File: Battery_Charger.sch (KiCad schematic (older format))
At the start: 48 parts, among them J8 USB_B_Micro, Q10 BC817, Q11 BC807, Q12 BSS138, Q13 BSS138, Q14 BSS138, Q9 BSS84, SW2 set_current, SW3 PWRON, U23 BQ24079RGT, U24 Holder 2x18650

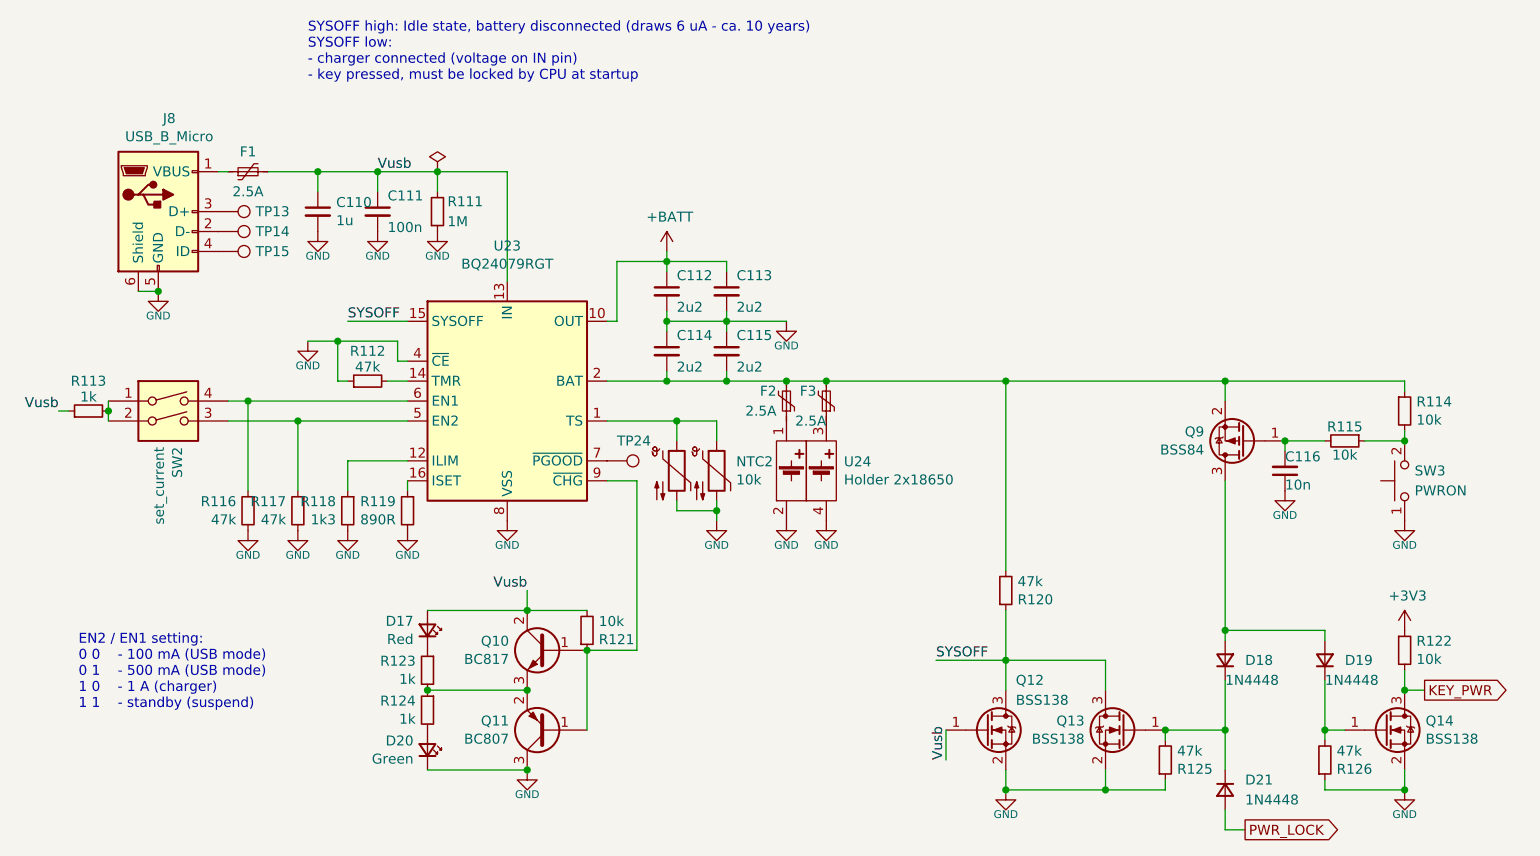
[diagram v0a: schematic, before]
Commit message: - PCB WiP
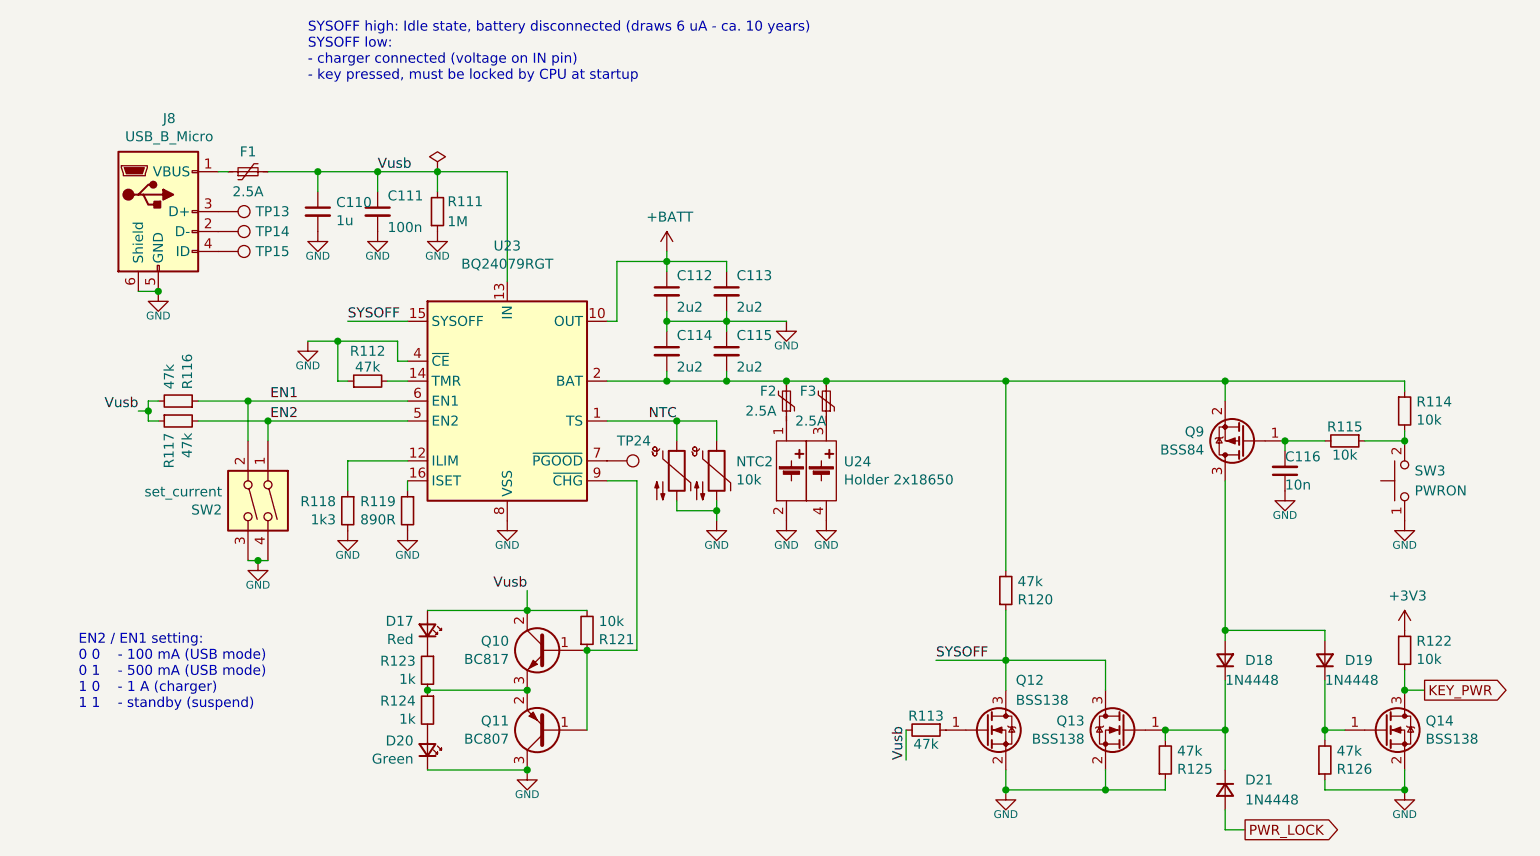
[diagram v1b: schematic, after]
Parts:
- D18, D19, D21: footprint Diode_SMD:D_SOD-323 -> miscellaneous_my:D_SOD-323-523_HandSoldering
- R113: value 1k -> 47k
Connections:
- net GND: now also SW2.3, SW2.4; no longer R116.2, R117.2
- net Vusb: now also R113.2, R116.2, R117.1; no longer Q12.1 (G), R113.1
- net NTC: now reaches NTC1.1, NTC2.1, U23.1 (TS)
- net EN1: now reaches R116.1, U23.6 (EN1)
- net EN1: now also SW2.2; no longer SW2.4
- new net: Q12.1 (G), R113.1
- new net EN2: R117.2, SW2.1, U23.5 (EN2)
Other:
- moved on the sheet: R116, R117, SW2
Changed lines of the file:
@@
 L Switch:SW_DIP_x02 SW?
 U 1 1 5F7AA902
-P 3150 3500
+P 3550 3900
 AR Path="/5F620813/5F7AA902" Ref="SW?"  Part="1"
 AR Path="/5F7A93EE/5F7AA902" Ref="SW2"  Part="1"
-F 0 "SW2" V 3196 3370 50  0000 R CNN
-F 1 "set_current" V 3105 3370 50  0000 R CNN
-F 2 "Button_Switch_SMD:SW_DIP_SPSTx02_Slide_6.7x6.64mm_W8.61mm_P2.54mm_LowProfile" H 3150 3500 50  0001 C CNN
-F 3 "~" H 3150 3500 50  0001 C CNN
-	1    3150 3500
-	1    0    0    -1
+F 0 "SW2" V 3596 3770 50  0000 R CNN
+F 1 "set_current" V 3505 3770 50  0000 R CNN
+F 2 "Button_Switch_SMD:SW_DIP_SPSTx02_Slide_6.7x6.64mm_W8.61mm_P2.54mm_LowProfile" H 3550 3900 50  0001 C CNN
+F 3 "~" H 3550 3900 50  0001 C CNN
+	1    3550 3900
+	0    1    1    0
 $EndComp
 Text Label 4200 2250 0    50   ~ 0
@@
 	4300 3200 4300 3100
 $Comp
-L power:GND #PWR?
-U 1 1 5F7AA94B
-P 3800 4050
-AR Path="/5F40DCB9/5F7AA94B" Ref="#PWR?"  Part="1"
-AR Path="/5F618AB9/5F7AA94B" Ref="#PWR?"  Part="1"
-AR Path="/5F7AA94B" Ref="#PWR?"  Part="1"
-AR Path="/5F620813/5F7AA94B" Ref="#PWR?"  Part="1"
-AR Path="/5F7A93EE/5F7AA94B" Ref="#PWR0134"  Part="1"
-F 0 "#PWR0134" H 3800 3890 50  0001 C CNN
-F 1 "GND" H 3800 3950 39  0000 C TNN
-F 2 "" H 3800 4050 50  0001 C CNN
-F 3 "" H 3800 4050 50  0001 C CNN
-	1    3800 4050
-	1    0    0    -1
-$EndComp
-$Comp
 L Device:R_Small R?
 U 1 1 5F7AA951
-P 3550 3950
+P 3200 3400
 AR Path="/5F620813/5F7AA951" Ref="R?"  Part="1"
 AR Path="/5F7A93EE/5F7AA951" Ref="R116"  Part="1"
-F 0 "R116" H 3609 3996 50  0000 L CNN
-F 1 "47k" H 3609 3905 50  0000 L CNN
-F 2 "Resistor_SMD:R_0603_1608Metric" H 3550 3950 50  0001 C CNN
-F 3 "~" H 3550 3950 50  0001 C CNN
-	1    3550 3950
-	-1   0    0    -1
+F 0 "R116" H 3259 3446 50  0000 L CNN
+F 1 "47k" H 3259 3355 50  0000 L CNN
+F 2 "Resistor_SMD:R_0603_1608Metric" H 3200 3400 50  0001 C CNN
+F 3 "~" H 3200 3400 50  0001 C CNN
+	1    3200 3400
+	0    1    -1   0
 $EndComp
 $Comp
 L power:GND #PWR?
 U 1 1 5F7AA958
-P 3550 4050
+P 3600 4200
 AR Path="/5F40DCB9/5F7AA958" Ref="#PWR?"  Part="1"
 AR Path="/5F618AB9/5F7AA958" Ref="#PWR?"  Part="1"
@@
 AR Path="/5F620813/5F7AA958" Ref="#PWR?"  Part="1"
 AR Path="/5F7A93EE/5F7AA958" Ref="#PWR0133"  Part="1"
-F 0 "#PWR0133" H 3550 3890 50  0001 C CNN
-F 1 "GND" H 3550 3950 39  0000 C TNN
-F 2 "" H 3550 4050 50  0001 C CNN
-F 3 "" H 3550 4050 50  0001 C CNN
-	1    3550 4050
-	1    0    0    -1
-$EndComp
-Wire Wire Line
-	4350 3500 3800 3500
-Wire Wire Line
-	3800 3500 3800 3850
+F 0 "#PWR0133" H 3600 4040 50  0001 C CNN
+F 1 "GND" H 3600 4100 39  0000 C TNN
+F 2 "" H 3600 4200 50  0001 C CNN
+F 3 "" H 3600 4200 50  0001 C CNN
+	1    3600 4200
+	1    0    0    -1
+$EndComp
 Wire Wire Line
 	4350 3400 3550 3400
 Wire Wire Line
-	3550 3400 3550 3850
+	3550 3400 3550 3600
 Wire Wire Line
 	4850 2250 4850 2800
-Wire Wire Line
-	3800 3500 3450 3500
-Connection ~ 3800 3500
-Wire Wire Line
-	3550 3400 3450 3400
 Connection ~ 3550 3400
-Text Label 2600 3450 2    50   ~ 0
+Text Label 3000 3450 2    50   ~ 0
 Vusb
 $Comp
 L Device:R_Small R?
 U 1 1 5F7AA968
-P 3800 3950
+P 3200 3500
 AR Path="/5F620813/5F7AA968" Ref="R?"  Part="1"
 AR Path="/5F7A93EE/5F7AA968" Ref="R117"  Part="1"
-F 0 "R117" H 3859 3996 50  0000 L CNN
-F 1 "47k" H 3859 3905 50  0000 L CNN
-F 2 "Resistor_SMD:R_0603_1608Metric" H 3800 3950 50  0001 C CNN
-F 3 "~" H 3800 3950 50  0001 C CNN
-	1    3800 3950
-	-1   0    0    -1
+F 0 "R117" H 3259 3546 50  0000 L CNN
+F 1 "47k" H 3259 3455 50  0000 L CNN
+F 2 "Resistor_SMD:R_0603_1608Metric" H 3200 3500 50  0001 C CNN
+F 3 "~" H 3200 3500 50  0001 C CNN
+	1    3200 3500
+	0    -1   1    0
 $EndComp
 $Comp
@@
 $EndComp
 Connection ~ 4450 4850
-$Comp
-L Device:R_Small R?
-U 1 1 5F7AA98C
-P 2750 3450
-AR Path="/5F620813/5F7AA98C" Ref="R?"  Part="1"
-AR Path="/5F7A93EE/5F7AA98C" Ref="R113"  Part="1"
-F 0 "R113" V 2900 3450 50  0000 C CNN
-F 1 "1k" V 2850 3450 50  0000 C BNN
-F 2 "Resistor_SMD:R_0603_1608Metric" H 2750 3450 50  0001 C CNN
-F 3 "~" H 2750 3450 50  0001 C CNN
-	1    2750 3450
-	0    -1   -1   0
-$EndComp
-Wire Wire Line
-	2850 3400 2850 3450
-Connection ~ 2850 3450
-Wire Wire Line
-	2850 3450 2850 3500
-Wire Wire Line
-	2650 3450 2600 3450
+Wire Wire Line
+	3050 3450 3000 3450
 Wire Wire Line
 	4350 3300 4250 3300
@@
 Wire Wire Line
 	7850 4850 7850 4700
-Text Label 7050 5200 1    50   ~ 0
+Text Label 6850 5200 1    50   ~ 0
 Vusb
-Wire Wire Line
-	7050 5200 7050 5050
 $Comp
 L power:+BATT #PWR?
@@
 F 0 "D21" V 8400 5450 50  0000 L CNN
 F 1 "1N4448" V 8500 5450 50  0000 L CNN
-F 2 "Diode_SMD:D_SOD-323" H 8450 5175 50  0001 C CNN
+F 2 "miscellaneous_my:D_SOD-323-523_HandSoldering" H 8450 5175 50  0001 C CNN
 F 3 "https://www.vishay.com/docs/81387/1n4448ws.pdf" H 8450 5350 50  0001 C CNN
 	1    8450 5350
@@
 F 0 "D18" V 8450 4600 50  0000 R CNN
 F 1 "1N4448" V 8350 4700 50  0000 R CNN
-F 2 "Diode_SMD:D_SOD-323" H 8450 4525 50  0001 C CNN
+F 2 "miscellaneous_my:D_SOD-323-523_HandSoldering" H 8450 4525 50  0001 C CNN
 F 3 "https://www.vishay.com/docs/81387/1n4448ws.pdf" H 8450 4700 50  0001 C CNN
 	1    8450 4700
@@
 F 0 "D19" V 8950 4600 50  0000 R CNN
 F 1 "1N4448" V 8850 4700 50  0000 R CNN
-F 2 "Diode_SMD:D_SOD-323" H 8950 4525 50  0001 C CNN
+F 2 "miscellaneous_my:D_SOD-323-523_HandSoldering" H 8950 4525 50  0001 C CNN
 F 3 "https://www.vishay.com/docs/81387/1n4448ws.pdf" H 8950 4700 50  0001 C CNN
 	1    8950 4700
@@
 	9150 3600 9350 3600
 Connection ~ 9350 3600
+Wire Wire Line
+	3050 3400 3050 3450
+Wire Wire Line
+	3550 4200 3600 4200
+Connection ~ 3600 4200
+Wire Wire Line
+	3600 4200 3650 4200
+Wire Wire Line
+	3650 3600 3650 3500
+Connection ~ 3650 3500
+Wire Wire Line
+	3650 3500 4350 3500
+Wire Wire Line
+	3300 3500 3650 3500
+Wire Wire Line
+	3300 3400 3550 3400
+Wire Wire Line
+	3100 3400 3050 3400
+Wire Wire Line
+	3100 3500 3050 3500
+Connection ~ 3050 3450
+Wire Wire Line
+	3050 3450 3050 3500
+$Comp
+L Device:R_Small R?
+U 1 1 5FB20FEF
+P 6950 5050
+AR Path="/5F7D6767/5FB20FEF" Ref="R?"  Part="1"
+AR Path="/5F7A93EE/5FB20FEF" Ref="R113"  Part="1"
+F 0 "R113" V 6850 5050 50  0000 C TNN
+F 1 "47k" V 7050 5050 50  0000 C BNN
+F 2 "Resistor_SMD:R_0603_1608Metric" H 6950 5050 50  0001 C CNN
+F 3 "~" H 6950 5050 50  0001 C CNN
+	1    6950 5050
+	0    1    1    0
+$EndComp
+Wire Wire Line
+	6850 5050 6850 5200
+Text Label 3800 3400 2    50   ~ 0
+EN1
+Text Label 3800 3500 2    50   ~ 0
+EN2
+Text Label 5700 3500 2    50   ~ 0
+NTC
 $EndSCHEMATC
